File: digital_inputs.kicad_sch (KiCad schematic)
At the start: 37 parts, among them U301 74HC595, U302 74HCT244

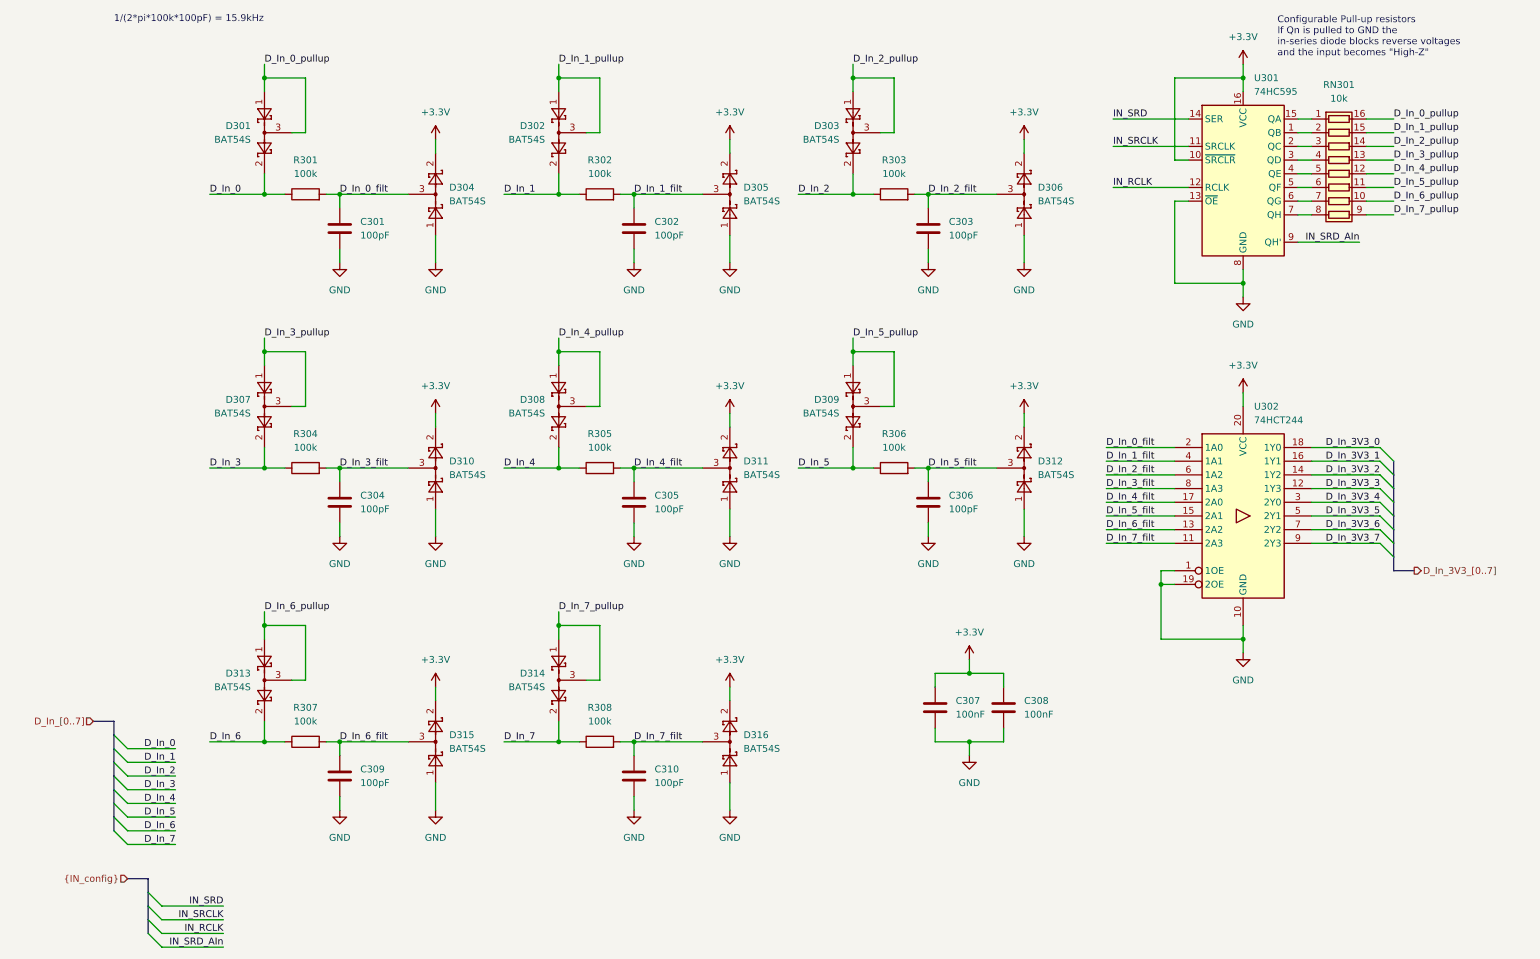
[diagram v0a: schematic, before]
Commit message: completed schematic
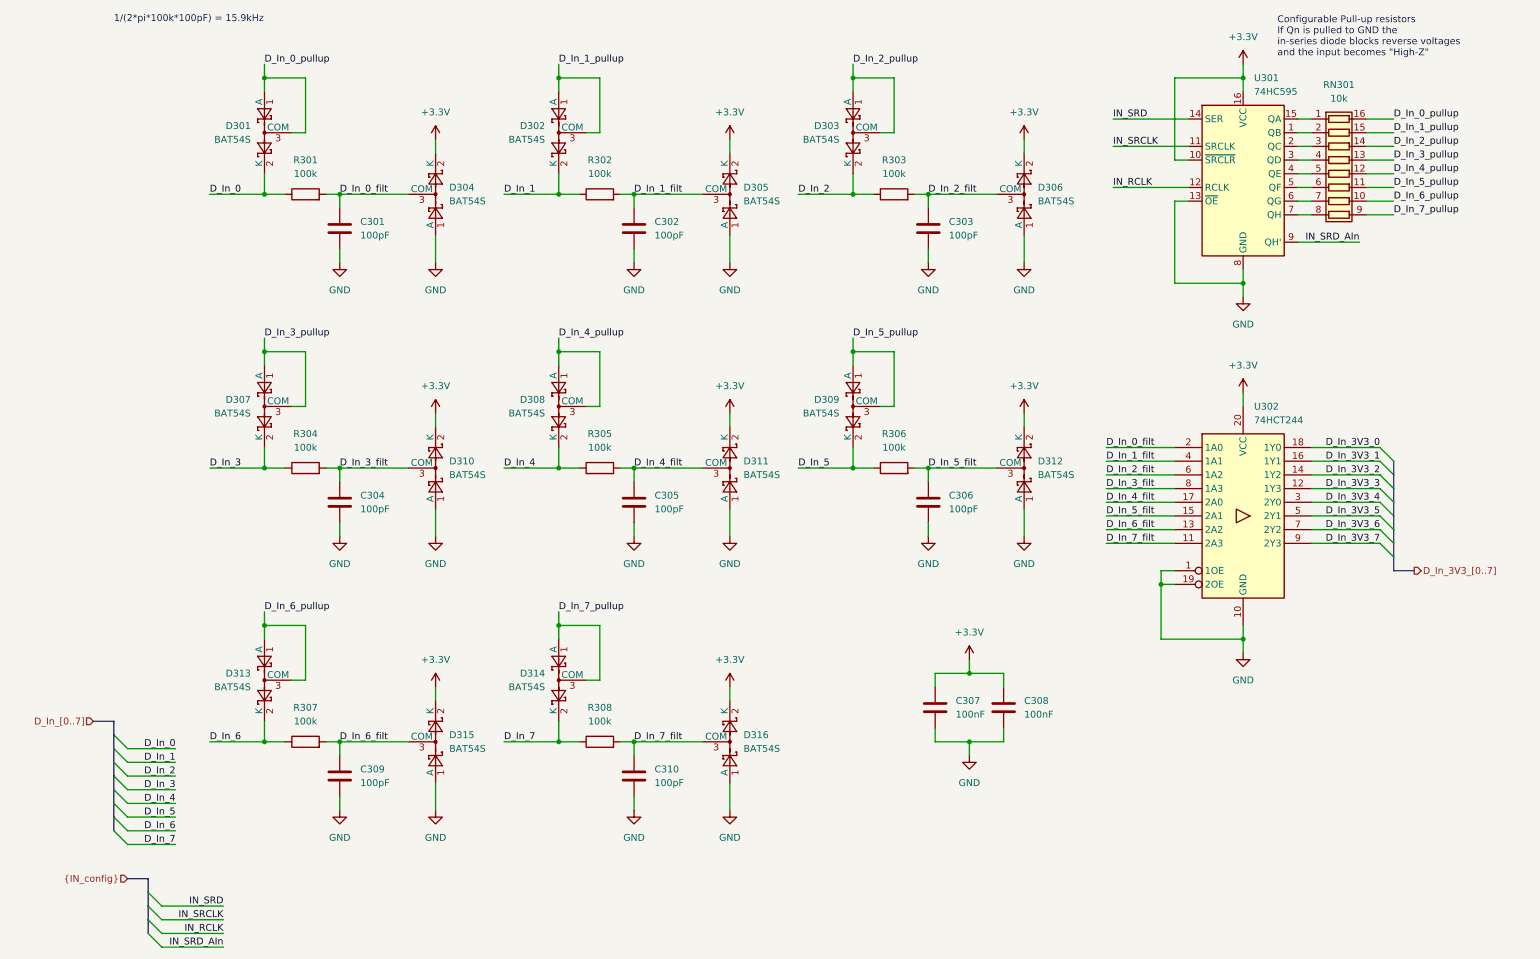
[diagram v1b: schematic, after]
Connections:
- net +3V3 renamed +3.3V
